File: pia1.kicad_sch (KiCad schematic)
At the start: 33 parts, among them IC20 MC14529B, IC24 74ACT244N, IC25 LM393P, U5 W65C21

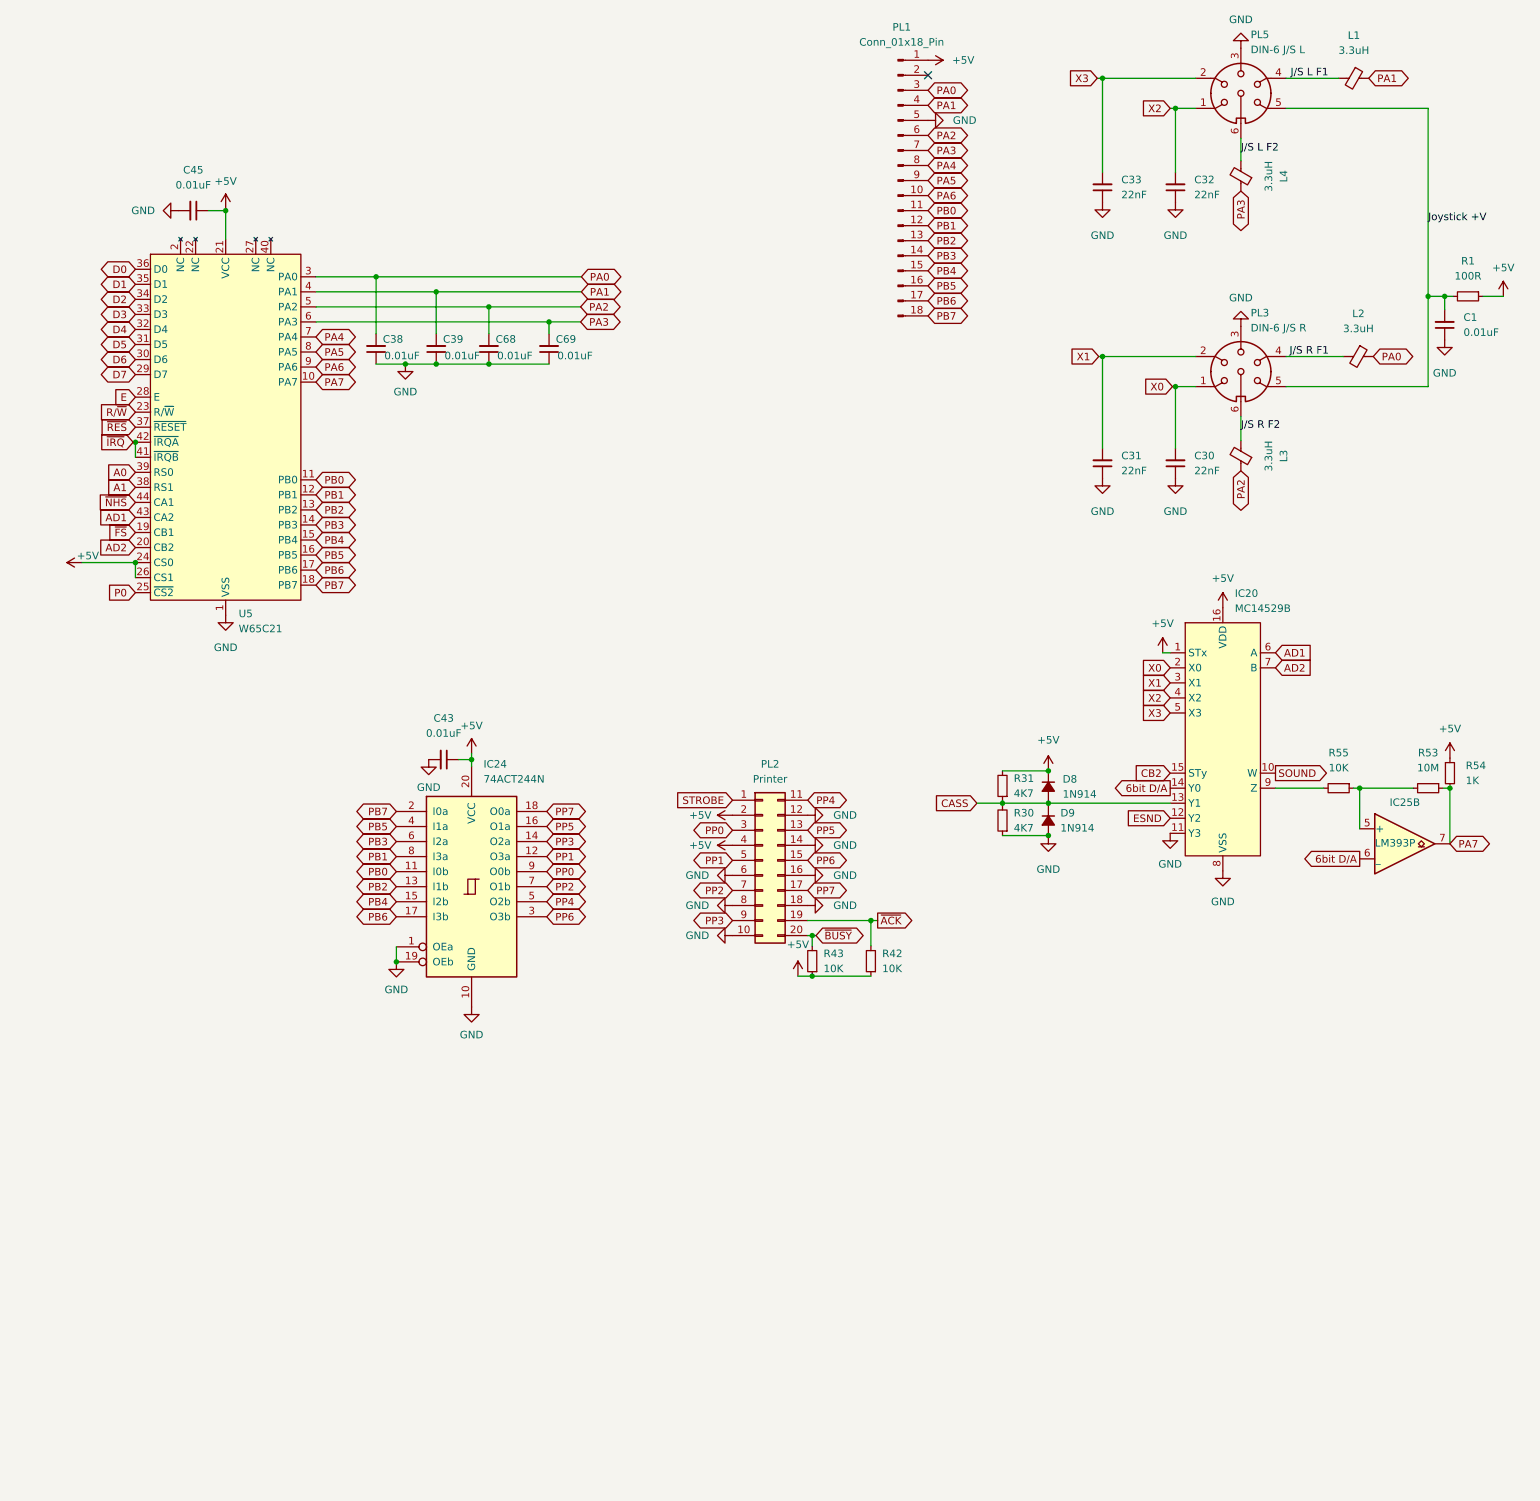
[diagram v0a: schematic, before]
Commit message: serial wiring
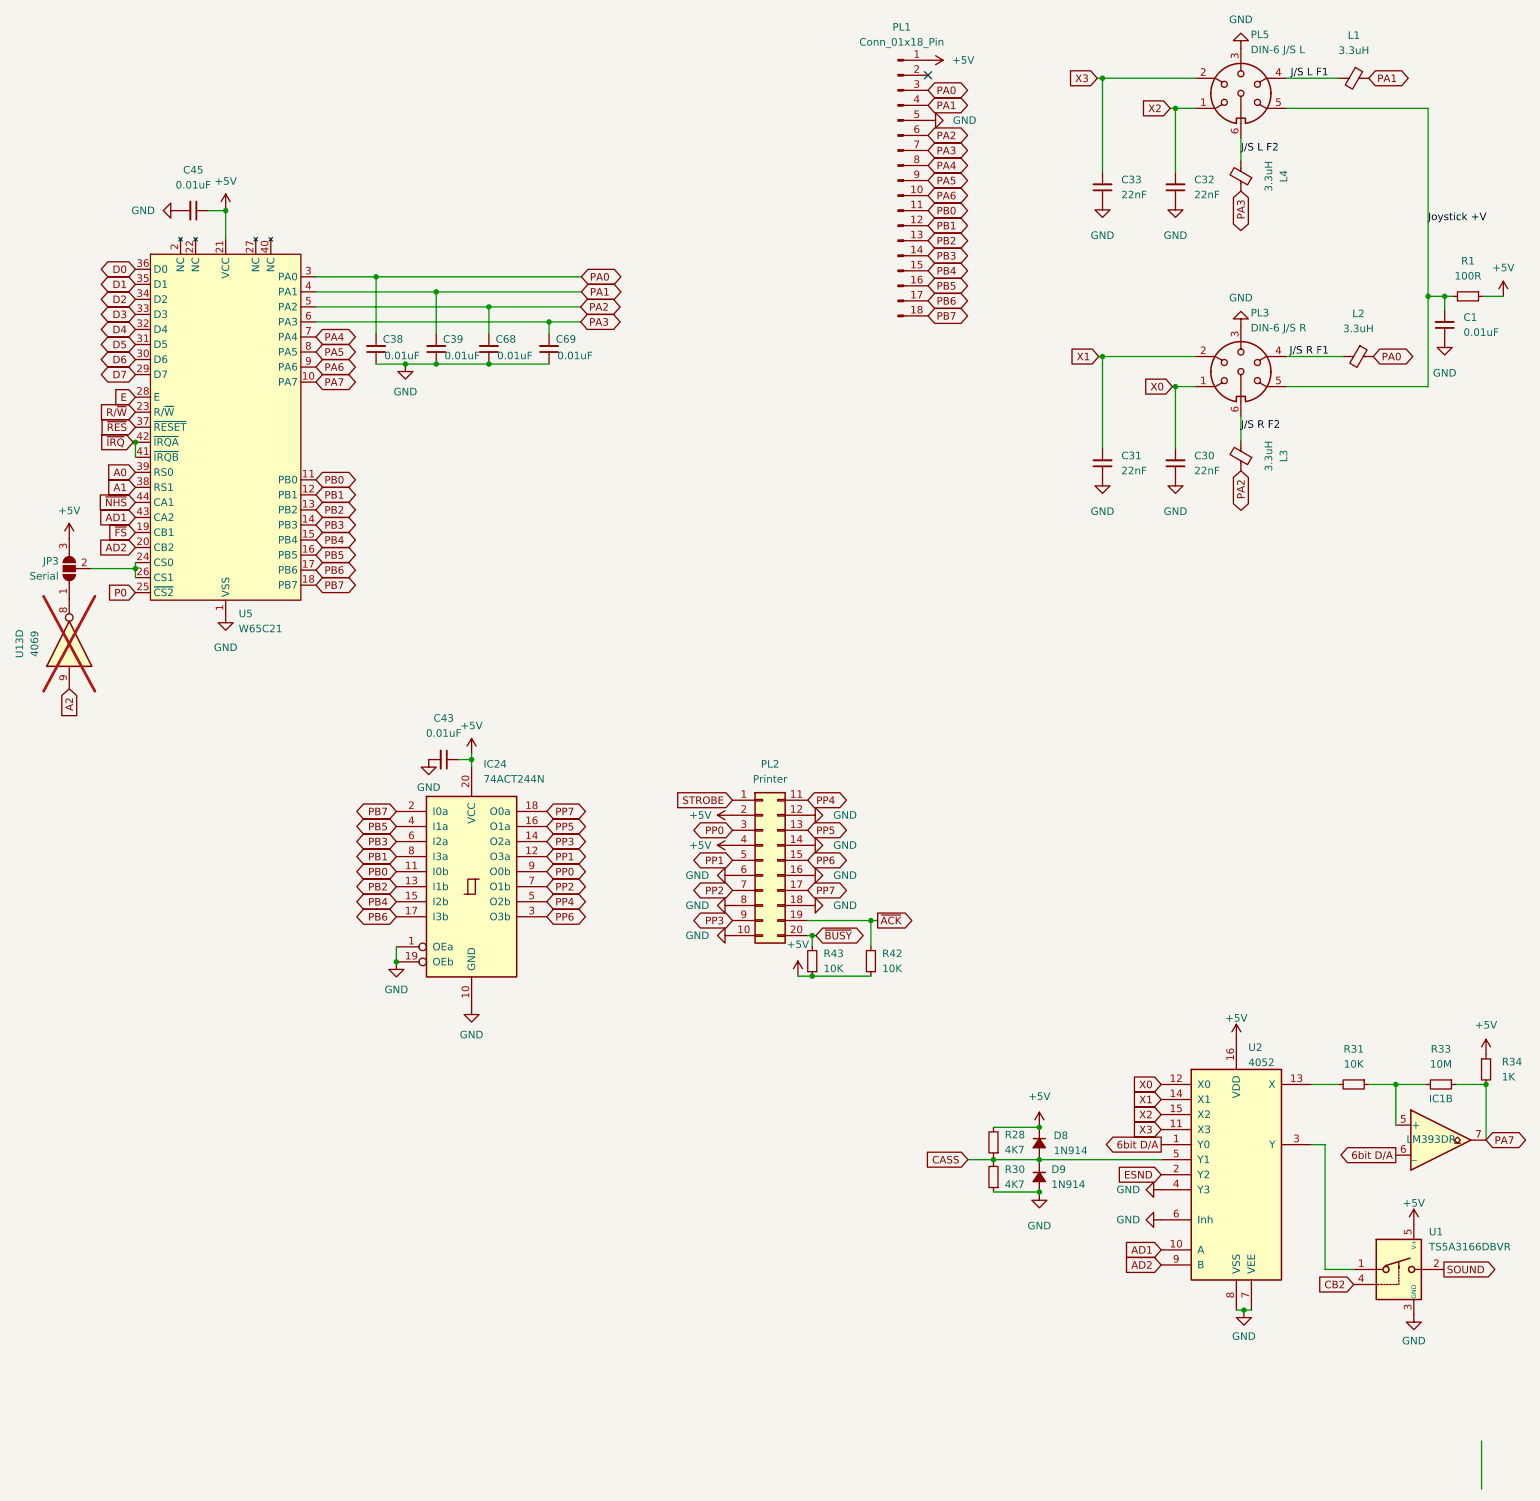
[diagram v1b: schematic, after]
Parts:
- removed IC20: MC14529B, Package_DIP:DIP-16_W7.62mm, symbol Motorola PIA:MC14529B
- removed IC25: LM393P, Package_DIP:DIP-8_W7.62mm, symbol Comparator:LM393
- removed R53: 10M, Resistor_SMD:R_0805_2012Metric_Pad1.20x1.40mm_HandSolder, symbol Device:R_Small
- removed R54: 1K, Resistor_SMD:R_0805_2012Metric_Pad1.20x1.40mm_HandSolder, symbol Device:R_Small
- removed R55: 10K, Resistor_SMD:R_0805_2012Metric_Pad1.20x1.40mm_HandSolder, symbol Device:R_Small
- added IC1: LM393DR, Package_SO:SOP-8_3.9x4.9mm_P1.27mm, symbol Comparator:LM393
- added JP3: Serial, Jumper:SolderJumper-3_P1.3mm_Open_Pad1.0x1.5mm, symbol Jumper:SolderJumper_3_Open
- added R28: 4K7, Resistor_SMD:R_0805_2012Metric_Pad1.20x1.40mm_HandSolder, symbol Device:R_Small
- added R33: 10M, Resistor_SMD:R_0805_2012Metric_Pad1.20x1.40mm_HandSolder, symbol Device:R_Small
- added R34: 1K, Resistor_SMD:R_0805_2012Metric_Pad1.20x1.40mm_HandSolder, symbol Device:R_Small
- added U1: TS5A3166DBVR, Package_TO_SOT_SMD:SOT-23-5, symbol Analog_Switch:TS5A3166DBVR
- added U13: 4069, Package_SO:SOIC-14_3.9x8.7mm_P1.27mm, symbol 4xxx:4069
- added U2: 4052, Package_SO:TSSOP-16_4.4x5mm_P0.65mm, symbol 4xxx:4052
- R31: value 4K7 -> 10K; DigiKey CF14JT4K70CT-ND -> CF14JT10K0CT-ND
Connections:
- net +5V: now also JP3.3 (B), R28.2, R34.1, U1.5 (V+), U2.16 (VDD); no longer R31.2, U5.24 (CS0), U5.26 (CS1)
- net 6bit D/A: now also IC1.6 (_), U2.1 (Y0)
- net AD1: now also U2.10 (A)
- net AD2: now also U2.9 (B)
- net CASS: now also R28.1, U2.5 (Y1); no longer R31.1
- net CB2: now also U1.4
- net ESND: now also U2.2 (Y2)
- net GND: now also U1.3 (GND), U2.4 (Y3), U2.6 (Inh), U2.7 (VEE), U2.8 (VSS)
- net PA7: now also IC1.7, R33.1, R34.2
- net SOUND: now also U1.2
- net X0: now also U2.12 (X0)
- net X1: now also U2.14 (X1)
- net X2: now also U2.15 (X2)
- net X3: now also U2.11 (X3)
- new net: JP3.1 (A), U13.8
- new net: JP3.2 (C), U5.24 (CS0), U5.26 (CS1)
- new net: IC1.5 (+), R31.1, R33.2
- new net: U1.1, U2.3 (Y)
- new net: R31.2, U2.13 (X)
- new net A2: U13.9
